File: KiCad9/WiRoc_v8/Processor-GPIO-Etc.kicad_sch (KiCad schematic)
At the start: 6 parts

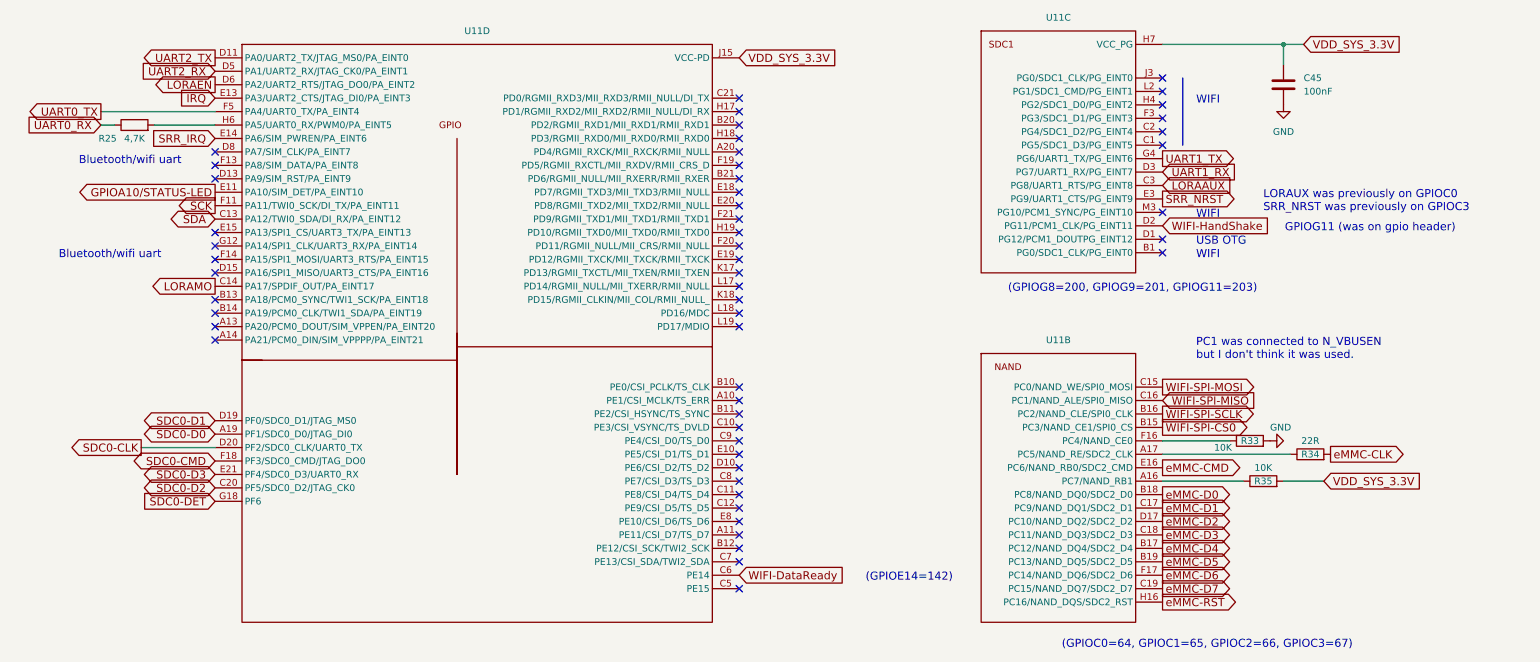
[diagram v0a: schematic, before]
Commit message: etc
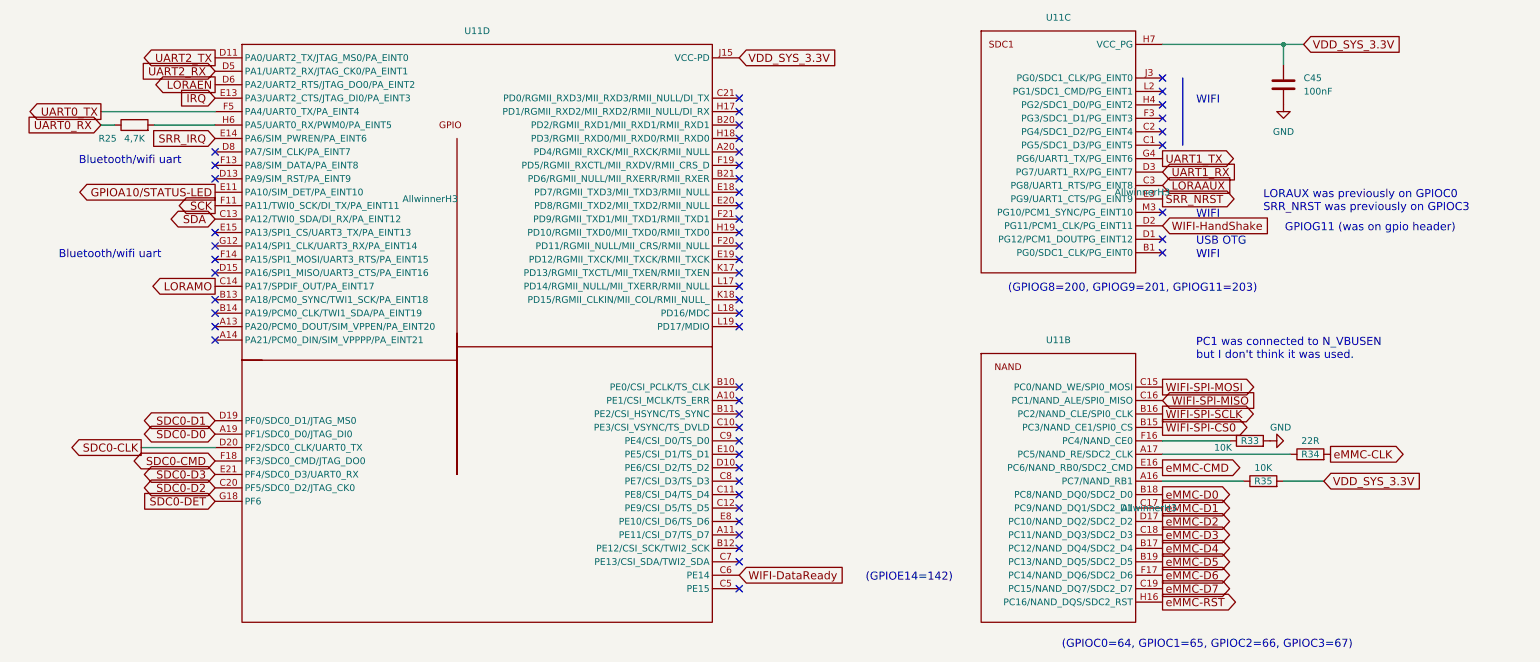
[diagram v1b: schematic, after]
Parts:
- R33, R35: LCSC Part # (none) -> C25804; Manufacturer (none) -> Uniroyal Elec; ManufacturerPartNumber (none) -> 0603WAF1002T5E
- U11: value ~ -> AllwinnerH3
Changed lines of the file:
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@@
 			)
 		)
-		(property "Value" "~"
+		(property "Value" "AllwinnerH3"
 			(at 96.52 68.58 0)
 			(effects
@@
 			)
 		)
-		(property "Value" "~"
+		(property "Value" "AllwinnerH3"
 			(at 232.41 127 0)
 			(effects
@@
 		(property "Description" ""
 			(at 254 121.92 0)
+			(effects
+				(font
+					(size 1.27 1.27)
+				)
+				(hide yes)
+			)
+		)
+		(property "LCSC Part #" "C25804"
+			(at 254 121.92 90)
+			(effects
+				(font
+					(size 1.27 1.27)
+				)
+				(hide yes)
+			)
+		)
+		(property "Manufacturer" "Uniroyal Elec"
+			(at 254 121.92 90)
+			(effects
+				(font
+					(size 1.27 1.27)
+				)
+				(hide yes)
+			)
+		)
+		(property "ManufacturerPartNumber" "0603WAF1002T5E"
+			(at 254 121.92 90)
 			(effects
 				(font
@@
 			)
 		)
+		(property "LCSC Part #" "C25804"
+			(at 251.46 114.3 90)
+			(effects
+				(font
+					(size 1.27 1.27)
+				)
+				(hide yes)
+			)
+		)
+		(property "Manufacturer" "Uniroyal Elec"
+			(at 251.46 114.3 90)
+			(effects
+				(font
+					(size 1.27 1.27)
+				)
+				(hide yes)
+			)
+		)
+		(property "ManufacturerPartNumber" "0603WAF1002T5E"
+			(at 251.46 114.3 90)
+			(effects
+				(font
+					(size 1.27 1.27)
+				)
+				(hide yes)
+			)
+		)
 		(pin "2"
 		)
@@
 			)
 		)
-		(property "Value" "~"
+		(property "Value" "AllwinnerH3"
 			(at 231.14 67.31 0)
 			(effects
